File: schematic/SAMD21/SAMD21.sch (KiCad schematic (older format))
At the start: 1 part, among them IC1 ATSAMD21G18A-AU

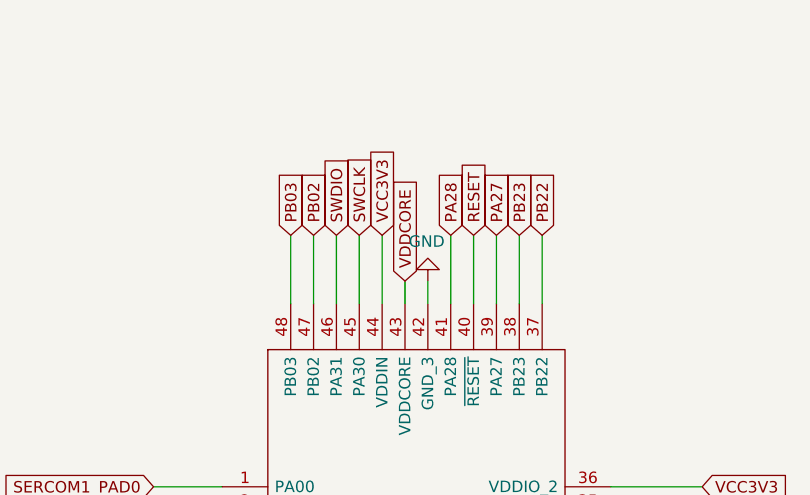
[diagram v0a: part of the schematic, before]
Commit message: minor fix
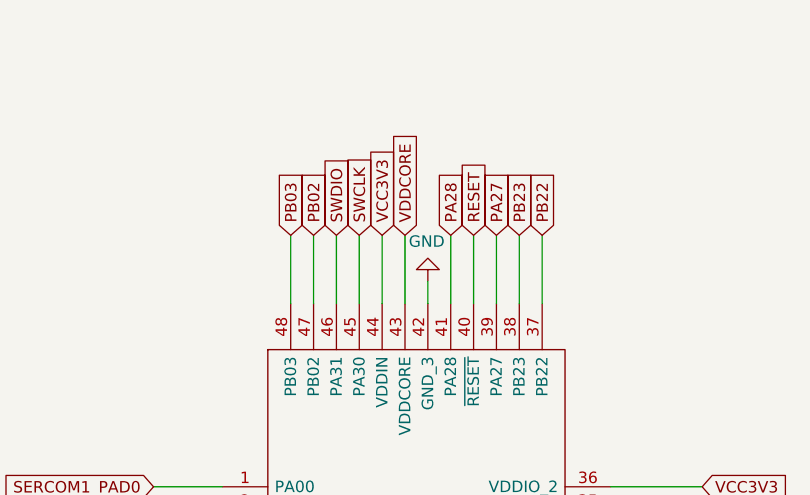
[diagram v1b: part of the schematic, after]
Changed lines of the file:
@@
 Wire Wire Line
 	6000 5000 6000 5350
-Text GLabel 5400 2200 1    50   Input ~ 0
+Text GLabel 5400 2000 1    50   Input ~ 0
 VDDCORE
-Wire Wire Line
-	5400 2300 5400 2200
 Text GLabel 4900 2000 1    50   Input ~ 0
 PB03
 Text GLabel 5000 2000 1    50   Input ~ 0
 PB02
+Wire Wire Line
+	5400 2000 5400 2300
 $EndSCHEMATC
